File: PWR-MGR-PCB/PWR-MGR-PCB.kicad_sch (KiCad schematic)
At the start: 0 parts

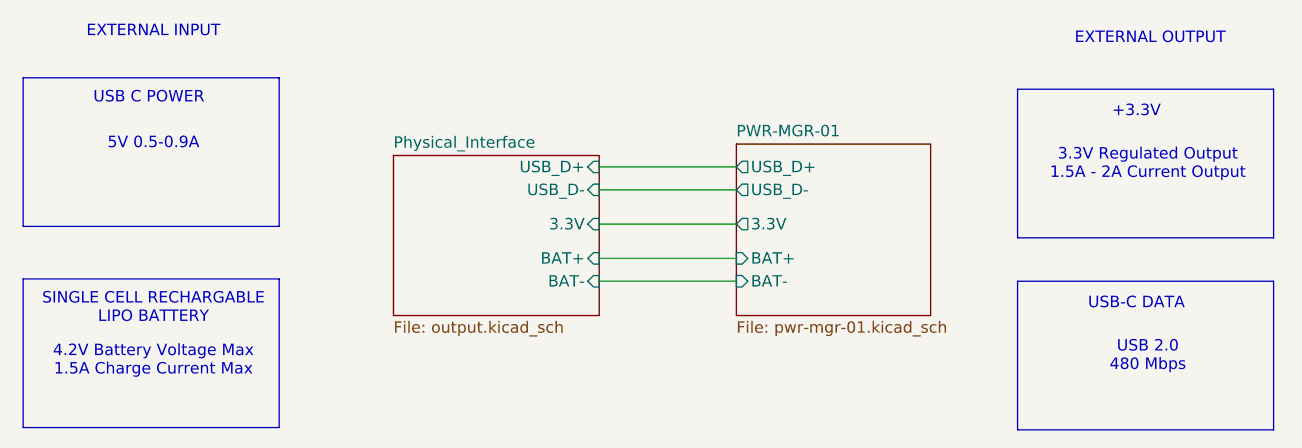
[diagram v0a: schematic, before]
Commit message: begin v2, update schematic
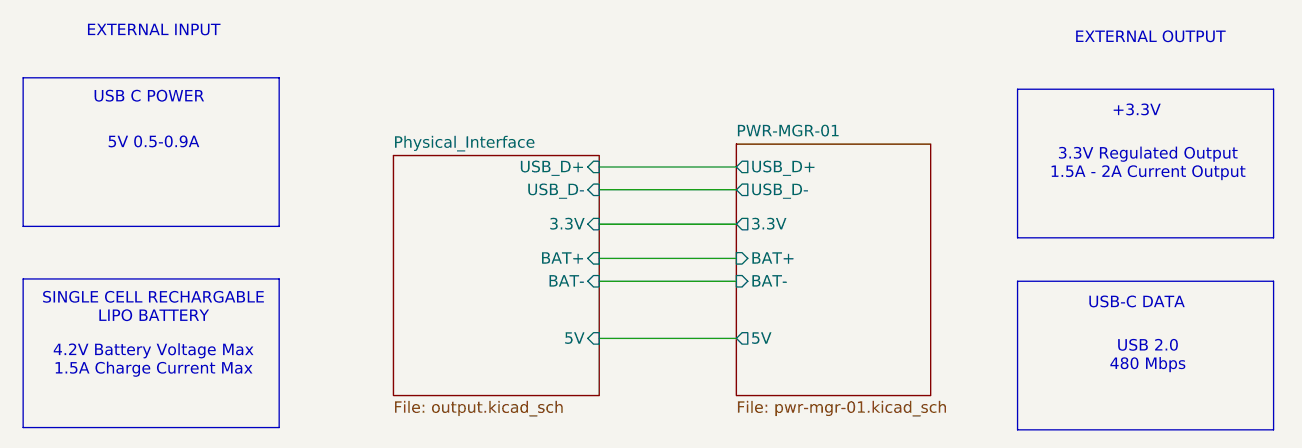
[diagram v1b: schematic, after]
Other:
- sheet PWR-MGR-01 ports: added 5V; removed none
- sheet Physical_Interface ports: added 5V; removed none
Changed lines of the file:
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@@
 (kicad_sch
-	(version 20250114)
+	(version 20260306)
 	(generator "eeschema")
-	(generator_version "9.0")
+	(generator_version "10.0")
 	(paper "A4")
 	(title_block
@@
 	(wire
 		(pts
+			(xy 148.59 106.68) (xy 163.83 106.68)
+		)
+		(stroke
+			(width 0)
+			(type default)
+		)
+	)
+	(wire
+		(pts
 			(xy 148.59 100.33) (xy 163.83 100.33)
 		)
@@
 	(sheet
 		(at 125.73 86.36)
-		(size 22.86 17.78)
+		(size 22.86 26.67)
 		(exclude_from_sim no)
 		(in_bom yes)
@@
 		)
 		(fill
-			(color 0 0 0 0.0000)
+			(color 0 0 0 0)
 		)
 		(property "Sheetname" "Physical_Interface"
 			(at 125.73 85.6484 0)
+			(show_name no)
+			(do_not_autoplace no)
 			(effects
 				(font
@@
 		)
 		(property "Sheetfile" "output.kicad_sch"
-			(at 125.73 104.7246 0)
+			(at 125.73 113.6146 0)
+			(show_name no)
+			(do_not_autoplace no)
 			(effects
 				(font
@@
 		(pin "BAT+" input
 			(at 148.59 97.79 0)
+			(effects
+				(font
+					(size 1.27 1.27)
+				)
+				(justify right)
+			)
+		)
+		(pin "5V" input
+			(at 148.59 106.68 0)
 			(effects
 				(font
@@
 	(sheet
 		(at 163.83 85.09)
-		(size 21.59 19.05)
+		(size 21.59 27.94)
 		(exclude_from_sim no)
 		(in_bom yes)
@@
 		)
 		(fill
-			(color 0 0 0 0.0000)
+			(color 0 0 0 0)
 		)
 		(property "Sheetname" "PWR-MGR-01"
 			(at 163.83 84.3784 0)
+			(show_name no)
+			(do_not_autoplace no)
 			(effects
 				(font
@@
 		)
 		(property "Sheetfile" "pwr-mgr-01.kicad_sch"
-			(at 163.83 104.7246 0)
+			(at 163.83 113.6146 0)
+			(show_name no)
+			(do_not_autoplace no)
 			(effects
 				(font
@@
 			(effects
 				(font
+					(size 1.27 1.27)
+				)
+				(justify left)
+			)
+		)
+		(pin "5V" output
+			(at 163.83 106.68 180)
+			(effects
+				(font
